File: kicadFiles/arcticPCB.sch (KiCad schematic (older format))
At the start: 175 parts, among them J1 TYPE-C-31-M12_13, J2 Conn_01x14, J3 Conn_ARM_JTAG_SWD_10, SW1 ESC, SW10 9, SW11 0, SW12 -_, SW13 +=, SW14 2U BKSP, SW15 TAB_150, SW16 Q, SW17 W, SW18 E, SW19 R, SW2 1, SW20 T, SW21 Y, SW22 U, SW23 I, SW24 O, SW25 P, SW26 [{, SW27 ]}, SW28 \\|_150, SW29 CAPS_175, SW3 2, SW30 A, SW31 S, SW32 D, SW33 F, SW34 G, SW35 H, SW36 J, SW37 K, SW38 L, SW39 :;, SW4 3, SW40 \"', SW41 ENTER_225, SW42 LSHIFT_225, SW43 Z, SW44 X, SW45 C, SW46 V, SW47 B, SW48 N, SW49 M, SW5 4, SW50 <,, SW51 >., SW52 ?/, SW53 RSHIFT_275, SW54 LCTRL_150, SW55 LGUI_100, SW56 LALT_150, SW57 SPACE_7U, SW58 RALT_150, SW59 RGUI_100, SW6 5, SW60 RCTRL_150, SW61 FN_100, SW62 RSHIFT_175, SW63 STEPPED_CAPS_125, SW64 1U LBKSP, SW65 1U RBKSP, SW7 6, SW8 7, SW9 8, U1 STM32F072-LQFP48, U2 USBLC6-2SC6, U3 MCP1700-3302E_SOT23

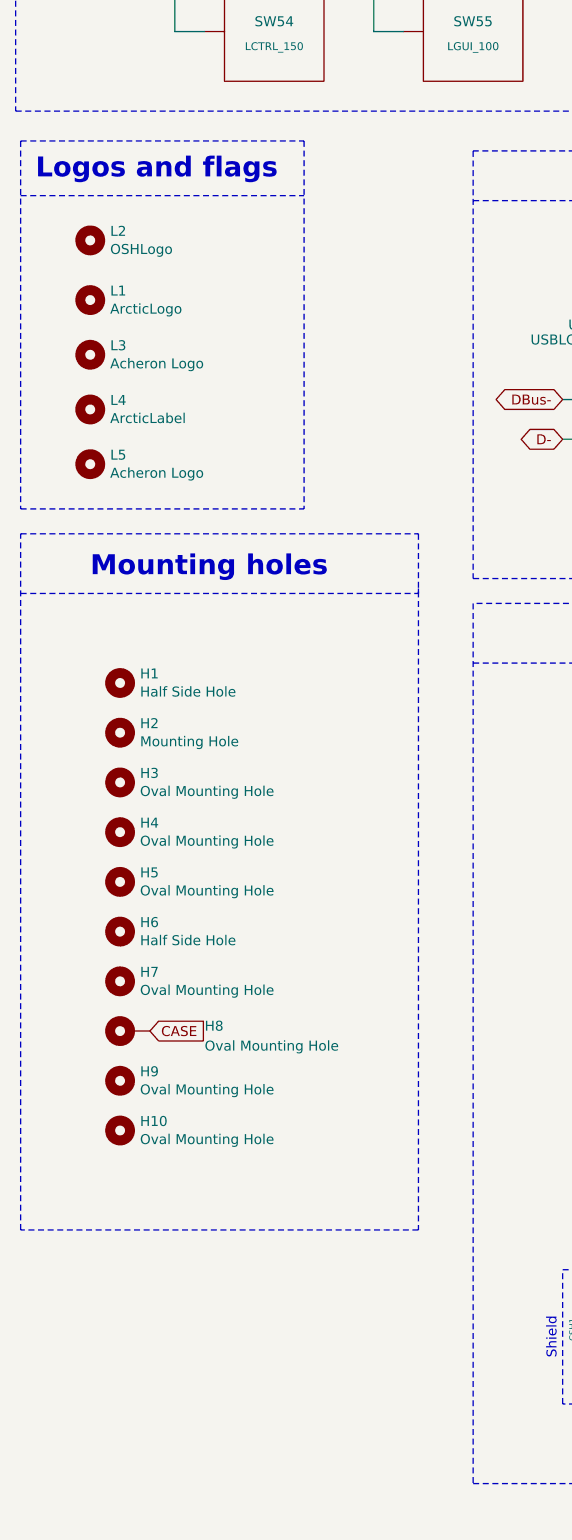
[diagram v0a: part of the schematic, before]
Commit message: Updated files and README
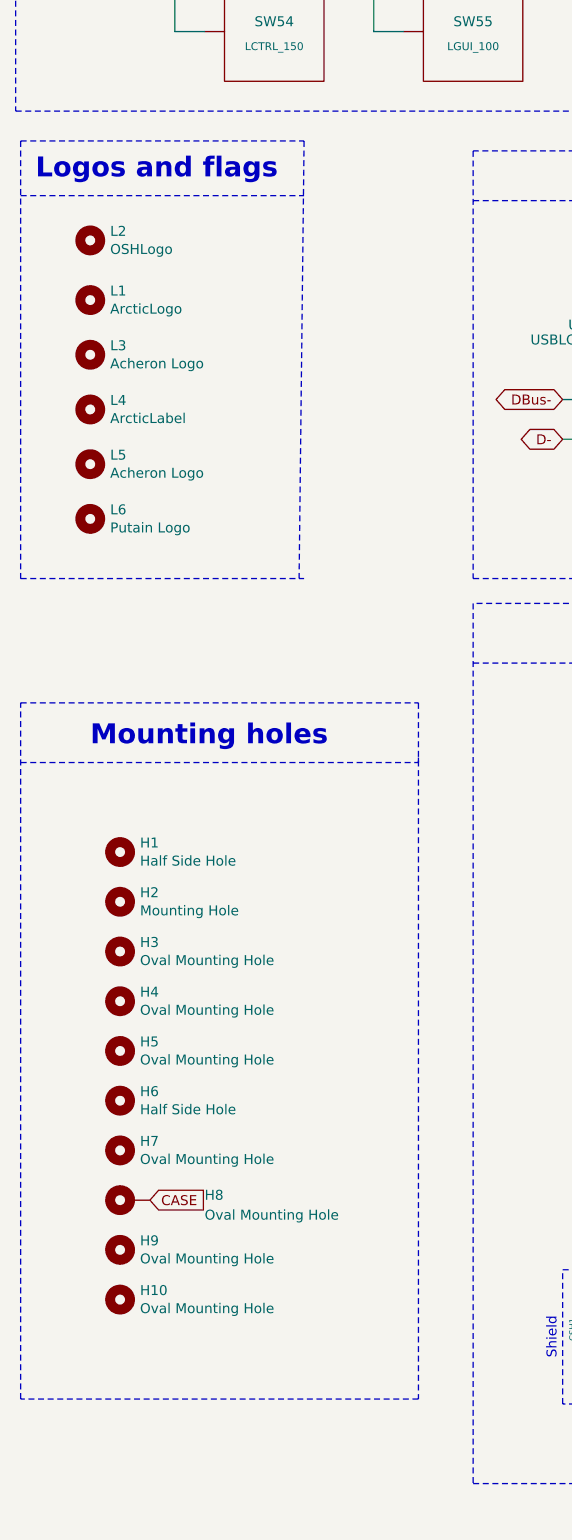
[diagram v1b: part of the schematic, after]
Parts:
- added L6: Putain Logo, arcticGraphics:putainLogo_50_5, symbol Mechanical:MountingHole
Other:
- moved on the sheet: H1, H10, H2, H3, H4, H5, H6, H7, H8, H9
